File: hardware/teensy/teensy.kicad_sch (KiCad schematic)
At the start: 26 parts, among them J1 CONN_16, J2 CONN_16, J3 CONN_04, U1 Teensy3.5

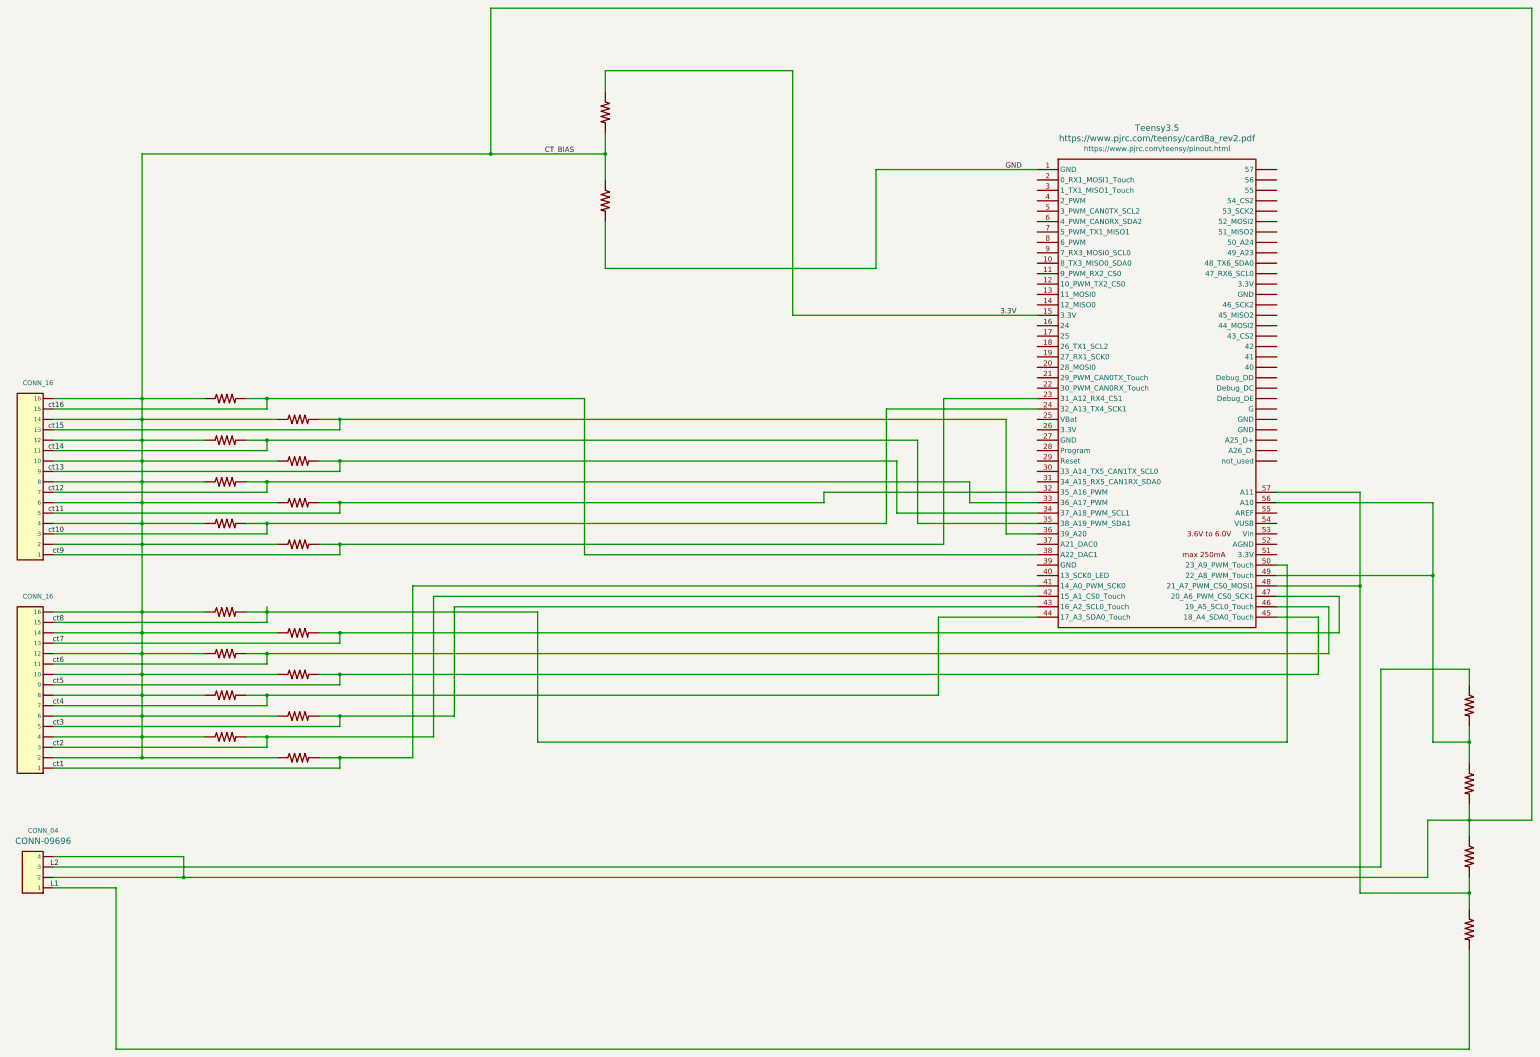
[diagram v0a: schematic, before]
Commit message: sch and pcb look good, also gbr and ngc outputs
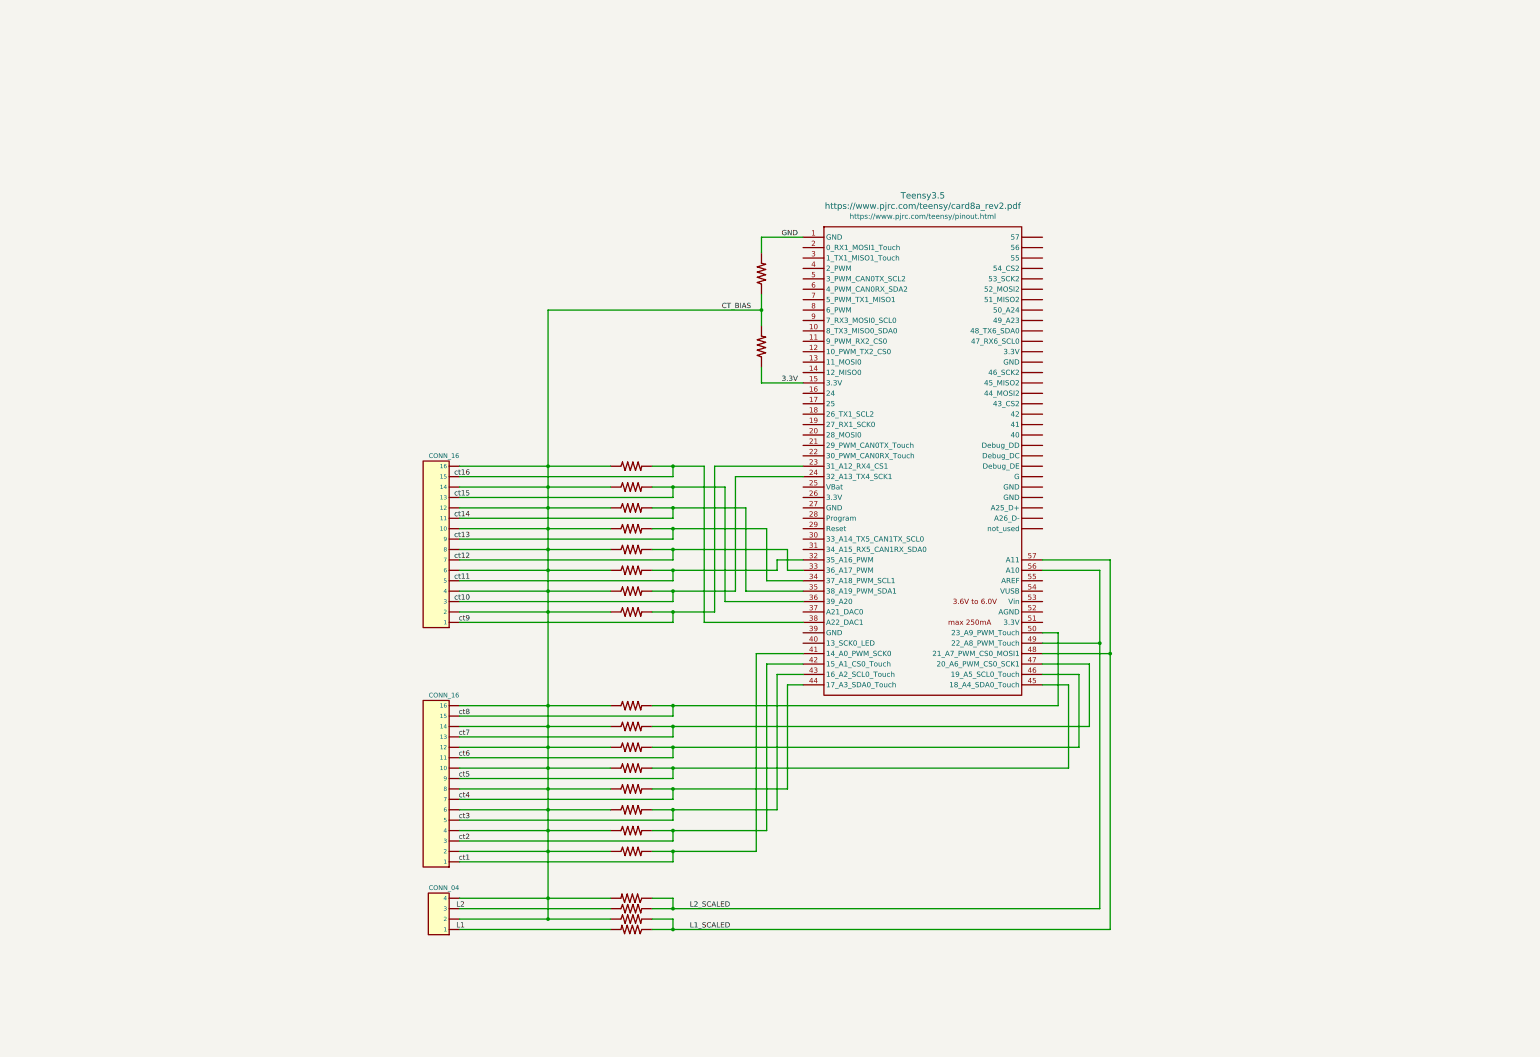
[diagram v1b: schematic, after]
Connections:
- net L2_SCALED: now reaches R19.P$2 (2), R20.P$1 (1), U1.49 (22_A8_PWM_Touch), U1.56 (A10)
- net L1_SCALED: now reaches R21.P$2 (2), R22.P$1 (1), U1.48 (21_A7_PWM_CS0_MOSI1), U1.57 (A11)
